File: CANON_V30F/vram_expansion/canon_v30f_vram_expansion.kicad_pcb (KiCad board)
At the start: 2 copper layers, 36.6 x 49 mm, 6 parts, among them IC1 DRAM_4464, IC2 DRAM_4464, J1 Conn_02x12_edgeconn_vram

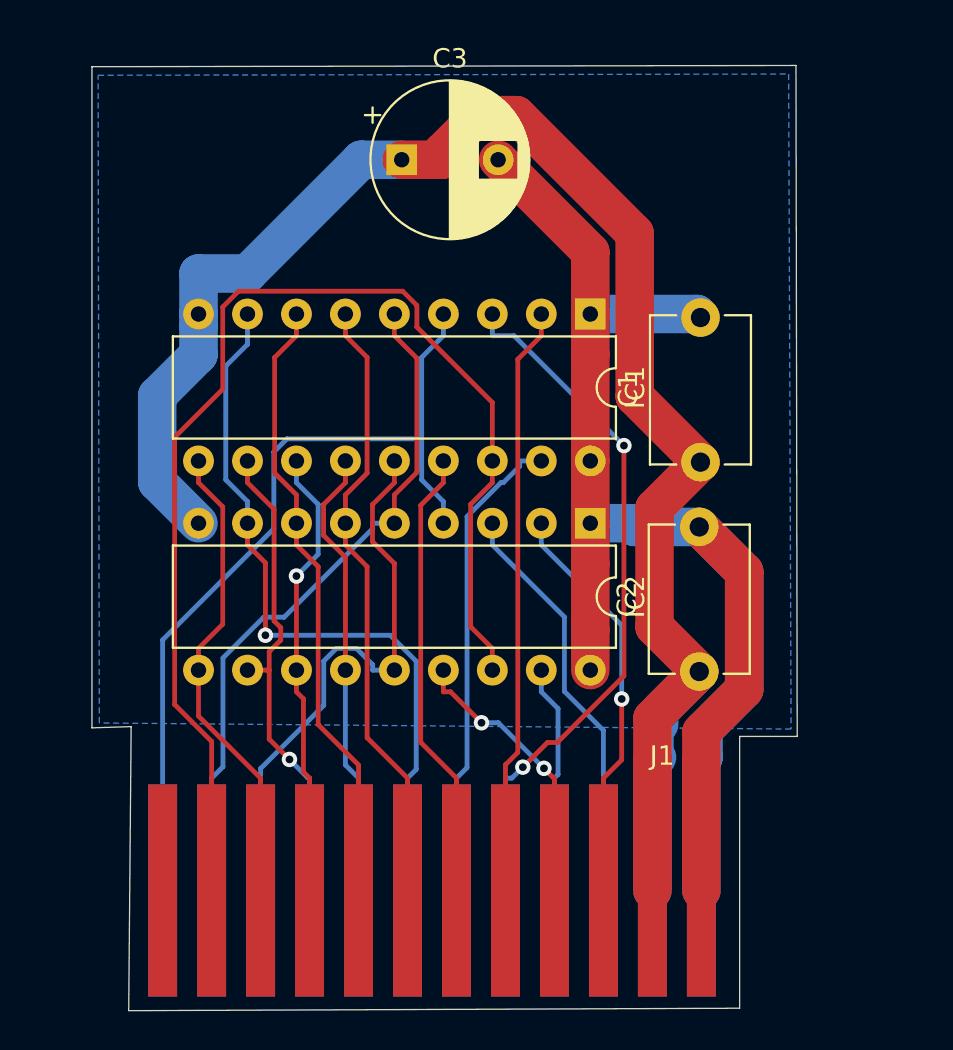
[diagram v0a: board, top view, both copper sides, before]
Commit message: Add files via upload
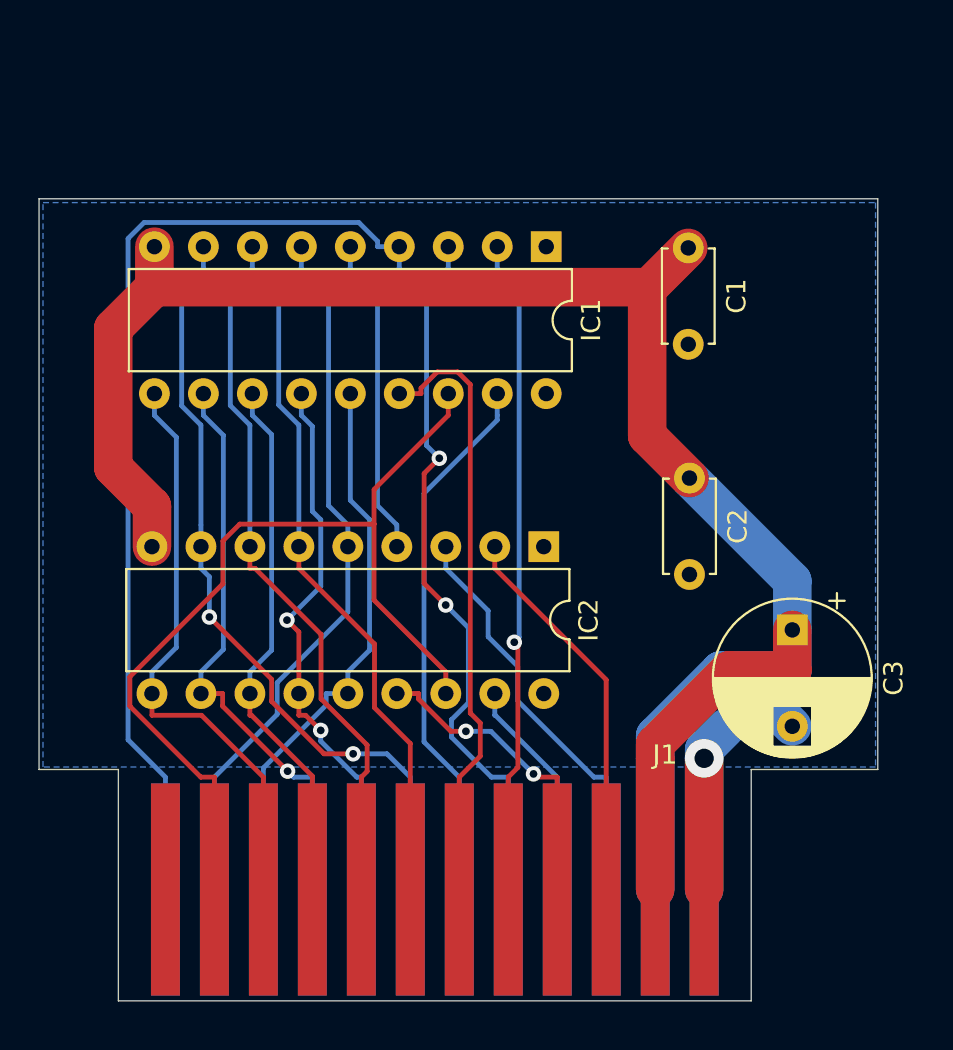
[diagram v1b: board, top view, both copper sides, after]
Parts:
- C1, C2: footprint Capacitor_THT:C_Disc_D7.5mm_W5.0mm_P7.50mm -> Capacitor_THT:C_Disc_D4.7mm_W2.5mm_P5.00mm
- moved C3 31.7 mm to (155.1, 86.4), turned to 270 degrees
- moved C1 11.1 mm to (149.7, 66.5), turned to 270 degrees
- moved C2 10.0 mm to (149.7, 78.5), turned to 270 degrees
- moved IC1 4.17 mm to (142.3, 66.5)
- moved IC2 2.70 mm to (142.2, 82.0)
- moved J1 0.15 mm to (136.5, 99.9)
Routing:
- net GND: track 81.4 -> 16.5 mm, vias 0 -> 1
- net _WE: track 44.9 -> 66.1 mm
- net _CAS1: track 64.3 -> 49.2 mm
- net +5V: track 94.4 -> 103.6 mm
- net 1_DQ3: track 23.5 -> 31.4 mm
- net A7: track 24.7 -> 30.6 mm
- net A1: track 23.5 -> 28.8 mm, vias 0 -> 2
- net A3: track 25.3 -> 30.3 mm
- net A5: track 32.2 -> 37.0 mm
- net A2: track 23.5 -> 28.0 mm, vias 1 -> 0
- net A6: track 32.2 -> 36.6 mm
- net 1_DQ1: track 30.7 -> 34.2 mm, vias 0 -> 1
- net 1_DQ4: track 24.8 -> 28.0 mm
- net A4: track 38.4 -> 40.6 mm, vias 1 -> 2
- net 2_DQ3: track 14.6 -> 16.1 mm
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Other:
- board size 36.6 x 49 mm -> 43.5 x 41.6 mm
